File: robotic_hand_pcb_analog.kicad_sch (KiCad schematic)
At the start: 36 parts, among them J10 A5, J11 A6, J12 A7, J13 ISENSE1, J14 ISENSE2, J15 ISENSE3, J16 ISENSE4, J17 ISENSE5, J6 A1, J7 A2, J8 A3, J9 A4, U10 ACS712xLCTR-05B, U11 ACS712xLCTR-05B, U12 ACS712xLCTR-05B, U13 ACS712xLCTR-05B, U8 ADS114S08, U9 ACS712xLCTR-05B

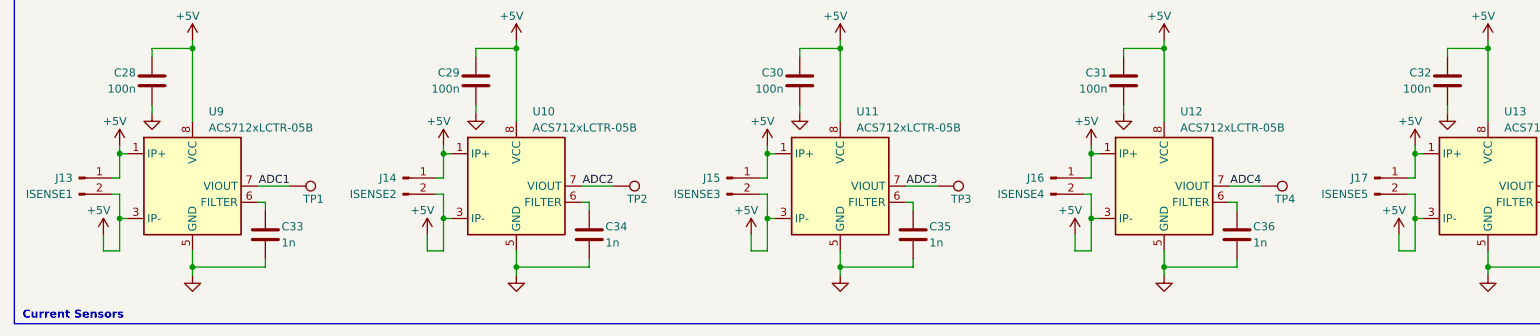
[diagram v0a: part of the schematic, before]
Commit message: Cleanup and remove unneeded connectors
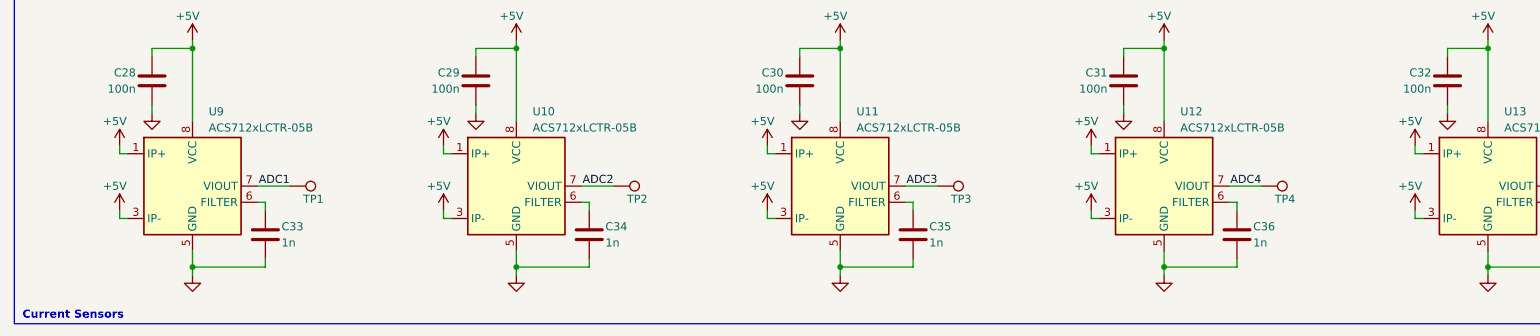
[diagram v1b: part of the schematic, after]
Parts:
- removed J13: ISENSE1, Connector_PinHeader_2.54mm:PinHeader_1x02_P2.54mm_Vertical, symbol Connector:Conn_01x02_Pin
- removed J14: ISENSE2, Connector_PinHeader_2.54mm:PinHeader_1x02_P2.54mm_Vertical, symbol Connector:Conn_01x02_Pin
- removed J15: ISENSE3, Connector_PinHeader_2.54mm:PinHeader_1x02_P2.54mm_Vertical, symbol Connector:Conn_01x02_Pin
- removed J16: ISENSE4, Connector_PinHeader_2.54mm:PinHeader_1x02_P2.54mm_Vertical, symbol Connector:Conn_01x02_Pin
- removed J17: ISENSE5, Connector_PinHeader_2.54mm:PinHeader_1x02_P2.54mm_Vertical, symbol Connector:Conn_01x02_Pin
